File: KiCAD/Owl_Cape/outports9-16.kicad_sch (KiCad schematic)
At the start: 36 parts, among them IC2 SN74HC244N, J10 G D V, J11 G D V, J12 G D V, J13 G D V, J14 G D V, J15 G D V, J16 G D V, J9 G D V

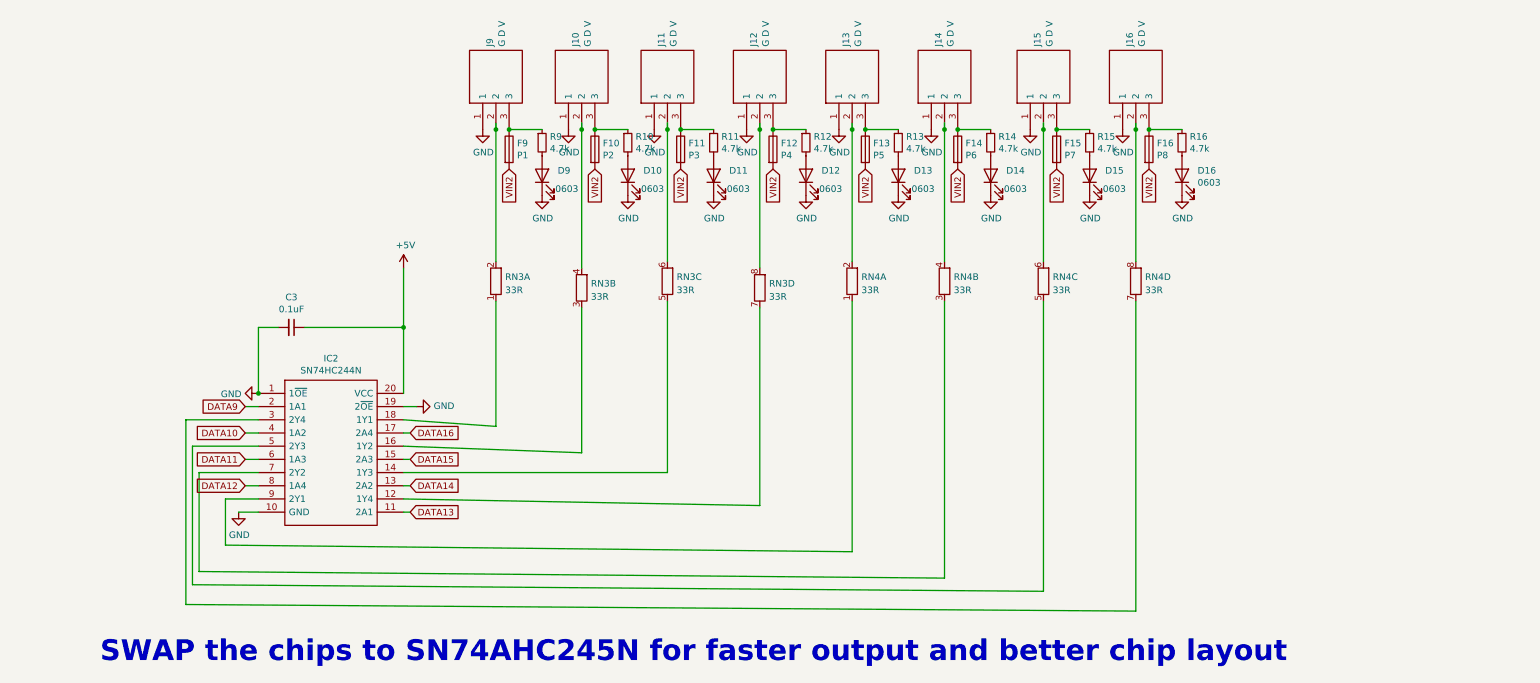
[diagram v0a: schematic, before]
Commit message: major update to layout
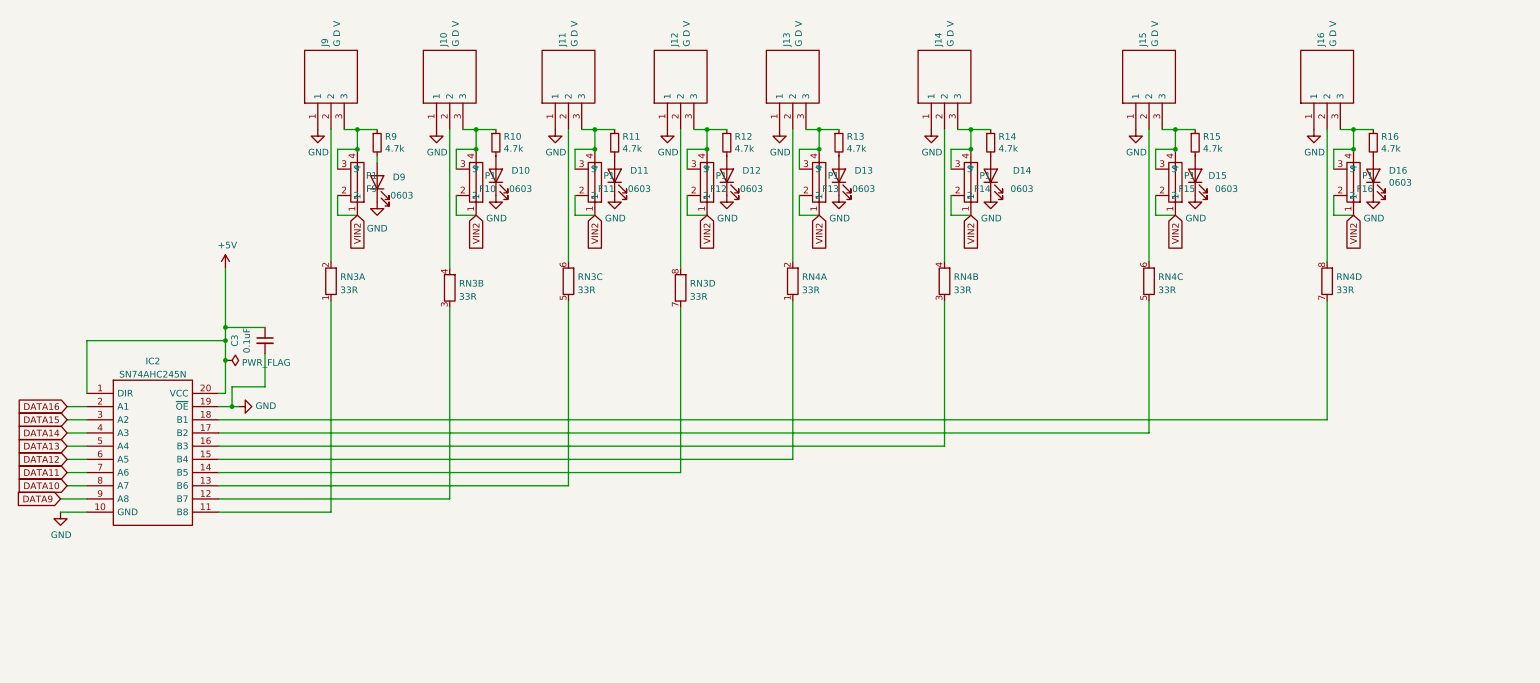
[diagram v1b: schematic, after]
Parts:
- removed F10: P2, Fuse:Fuseholder_Blade_Mini_Keystone_3568, symbol Device:Fuse
- removed F11: P3, Fuse:Fuseholder_Blade_Mini_Keystone_3568, symbol Device:Fuse
- removed F12: P4, Fuse:Fuseholder_Blade_Mini_Keystone_3568, symbol Device:Fuse
- removed F13: P5, Fuse:Fuseholder_Blade_Mini_Keystone_3568, symbol Device:Fuse
- removed F14: P6, Fuse:Fuseholder_Blade_Mini_Keystone_3568, symbol Device:Fuse
- removed F15: P7, Fuse:Fuseholder_Blade_Mini_Keystone_3568, symbol Device:Fuse
- removed F16: P8, Fuse:Fuseholder_Blade_Mini_Keystone_3568, symbol Device:Fuse
- removed F9: P1, Fuse:Fuseholder_Blade_Mini_Keystone_3568, symbol Device:Fuse
- removed IC2: SN74HC244N, SamacSys_Parts:DIP794W53P254L2540H508Q20N, symbol owl_cape-rescue:SN74HC244N-SamacSys_Parts
- added F10, F11, F12, F13, F14, F15, F16, F9: P1, Stuart_BESPOKE:Medium Auto Fuse Holder, symbol Stuarts_BESPOKE:Medium_Auto_Fuse_Holder
- added IC2: SN74AHC245N, DIP794W53P254L2540H508Q20N, symbol SamacSys_Parts:SN74AHC245N
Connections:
- net +5V: now also IC2.1 (DIR), IC2.20 (VCC)
- net DATA10: now also IC2.8 (A7)
- net DATA11: now also IC2.7 (A6)
- net DATA12: now also IC2.6 (A5)
- net DATA13: now also IC2.5 (A4)
- net DATA14: now also IC2.4 (A3)
- net DATA15: now also IC2.3 (A2)
- net DATA16: now also IC2.2 (A1)
- net DATA9: now also IC2.9 (A8)
- net GND: now also IC2.10 (GND), IC2.19 (~{OE})
- net VIN2: now also F10.1, F10.2, F11.1, F11.2, F12.1, F12.2, F13.1, F13.2, F14.1, F14.2, F15.1, F15.2, F16.1, F16.2, F9.1, F9.2
- net at J9.3, R9.1: now also F9.3, F9.4
- net at J10.3, R10.1: now also F10.3, F10.4
- net at J11.3, R11.1: now also F11.3, F11.4
- net at J12.3, R12.1: now also F12.3, F12.4
- net at J13.3, R13.1: now also F13.3, F13.4
- net at J14.3, R14.1: now also F14.3, F14.4
- net at J15.3, R15.1: now also F15.3, F15.4
- net at J16.3, R16.1: now also F16.3, F16.4
- net at RN3.7 (R4.1): now also IC2.14 (B5)
- net at RN3.5 (R3.1): now also IC2.13 (B6)
- net at RN3.3 (R2.1): now also IC2.12 (B7)
- net at RN3.1 (R1.1): now also IC2.11 (B8)
- net at RN4.7 (R4.1): now also IC2.18 (B1)
- net at RN4.5 (R3.1): now also IC2.17 (B2)
- net at RN4.3 (R2.1): now also IC2.16 (B3)
- net at RN4.1 (R1.1): now also IC2.15 (B4)
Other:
- note removed: "SWAP the chips to SN74AHC245N for faster output and better chip layout"
- moved on the sheet: C3, D10, D11, D12, D13, D15, D16, D9, J10, J11, J12, J13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
